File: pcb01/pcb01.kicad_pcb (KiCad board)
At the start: 2 copper layers, 7 parts, among them U1 W65C02SxP, U2 HM62256BLP, U3 27C512, U4 PAL20RS10, U5 74LS138, U6 74HCT574, U7 HM62256BLP

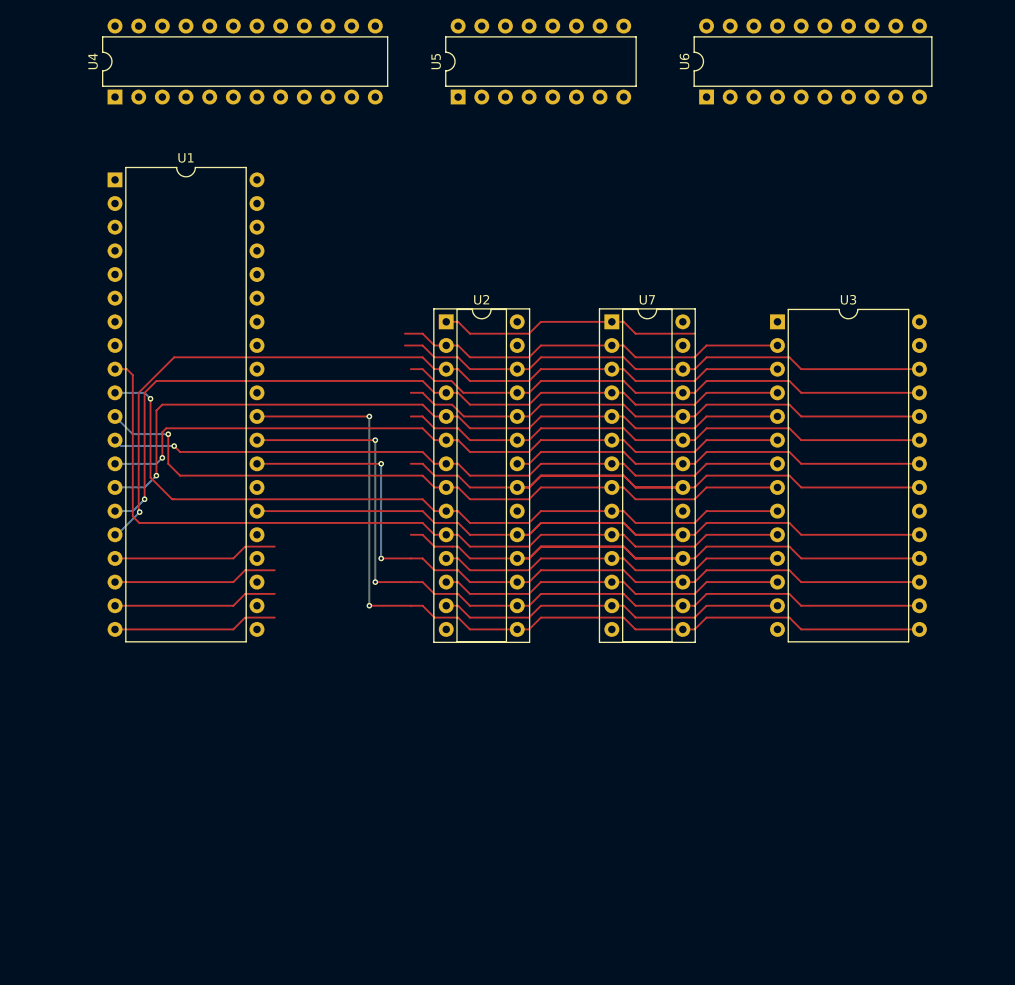
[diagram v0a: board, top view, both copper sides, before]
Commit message: more work on pcd layout
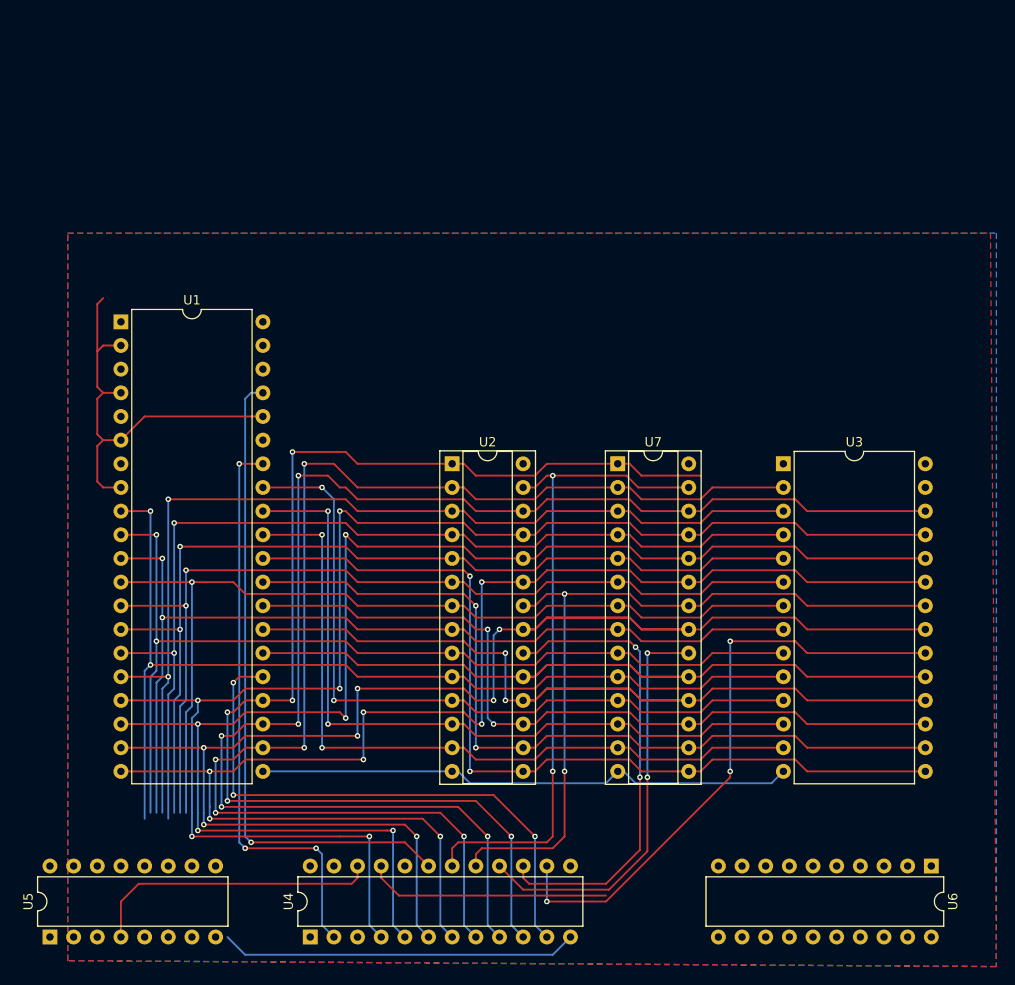
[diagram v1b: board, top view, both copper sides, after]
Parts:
- moved U5 100.3 mm to (13.3, 127.0)
- moved U4 92.6 mm to (41.3, 127.0)
- moved U6 86.0 mm to (108.0, 119.4), turned to -90 degrees
- moved U1 15.3 mm to (21.0, 61.0)
- moved U2 15.3 mm to (56.5, 76.2)
- moved U3 15.3 mm to (92.1, 76.2)
- moved U7 15.3 mm to (74.3, 76.2)
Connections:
- U3 pad 20: /CS_ROM -> /~{CS_ROM}
- U4 pad 16: /~{IO_SEL} -> /~{CS_RAM1}
- U4 pad 22: /~{CS_RAM1} -> /~{IO_SEL}
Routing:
- net /A14: track 28.3 -> 133.0 mm, vias 0 -> 5
- net /A12: track 42.6 -> 139.9 mm, vias 0 -> 5
- net /A13: track 58.4 -> 155.3 mm, vias 0 -> 5
- net GND: track 0.00 -> 96.4 mm
- net /A8: track 75.4 -> 154.3 mm, vias 0 -> 5
- net /A9: track 75.4 -> 154.3 mm, vias 0 -> 5
- net /A11: track 75.4 -> 151.8 mm, vias 0 -> 7
- net /~{QWE_RAM}: track 0.00 -> 70.8 mm, vias 0 -> 2
- net /SYS_CLK: track 0.00 -> 70.2 mm, vias 0 -> 1
- net /A10: track 94.3 -> 163.6 mm, vias 0 -> 7
- net /~{CS_ROM}: track 0.00 -> 65.7 mm, vias 0 -> 3
- net /R/~{W}: track 0.00 -> 62.0 mm, vias 0 -> 3
- net /A15: track 0.00 -> 61.1 mm, vias 0 -> 3
- net /~{CS_RAM0}: track 0.00 -> 50.4 mm, vias 0 -> 2
- net VCC: track 0.00 -> 46.7 mm
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- added copper zone on B.Cu, net GND
- added copper zone on F.Cu, net GND
